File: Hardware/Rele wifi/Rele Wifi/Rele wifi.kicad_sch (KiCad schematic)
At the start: 15 parts, among them J1 Screw_Terminal_01x02, J2 Screw_Terminal_01x03, K1 G5LE-1, Q1 BC337, Q2 BC337, U5 PC817

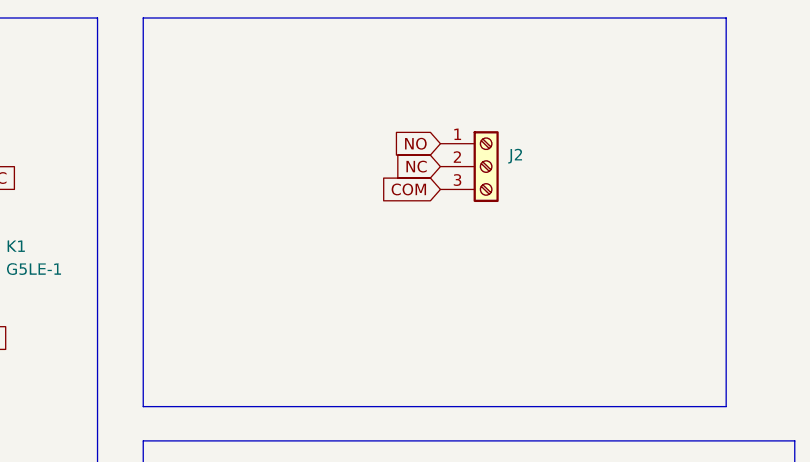
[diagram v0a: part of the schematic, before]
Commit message: act placa
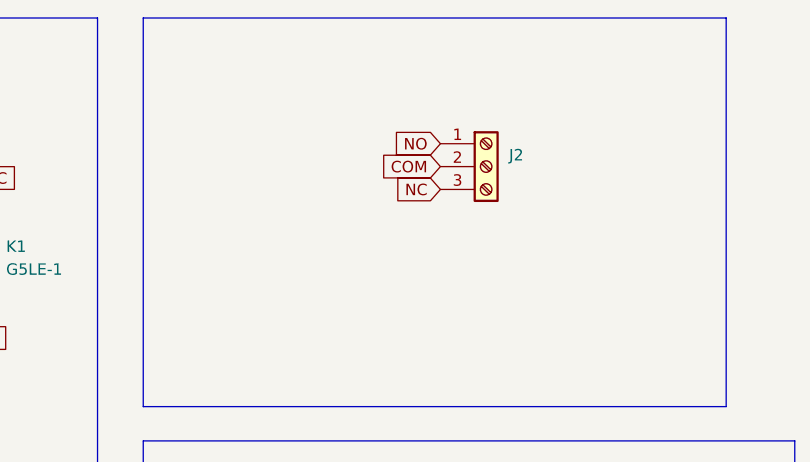
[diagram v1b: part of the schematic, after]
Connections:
- net COM: now also J2.2 (Pin_2); no longer J2.3 (Pin_3)
- net NC: now also J2.3 (Pin_3); no longer J2.2 (Pin_2)
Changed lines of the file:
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@@
 	(global_label "NC"
 		(shape input)
-		(at 234.95 30.48 180)
+		(at 234.95 33.02 180)
 		(fields_autoplaced yes)
 		(effects
@@
 		)
 		(property "Intersheetrefs" "${INTERSHEET_REFS}"
-			(at 229.3643 30.48 0)
+			(at 229.3643 33.02 0)
 			(effects
 				(font
@@
 	(global_label "COM"
 		(shape input)
-		(at 234.95 33.02 180)
+		(at 234.95 30.48 180)
 		(fields_autoplaced yes)
 		(effects
@@
 		)
 		(property "Intersheetrefs" "${INTERSHEET_REFS}"
-			(at 227.9129 33.02 0)
+			(at 227.9129 30.48 0)
 			(effects
 				(font
